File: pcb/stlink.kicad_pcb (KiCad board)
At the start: 4 copper layers, 36.5 x 20 mm, 41 parts, among them J1 USB_A, Q1 S9013, U1 XC6206P332MR, U2 STM32F103C8, Y1 8MHz

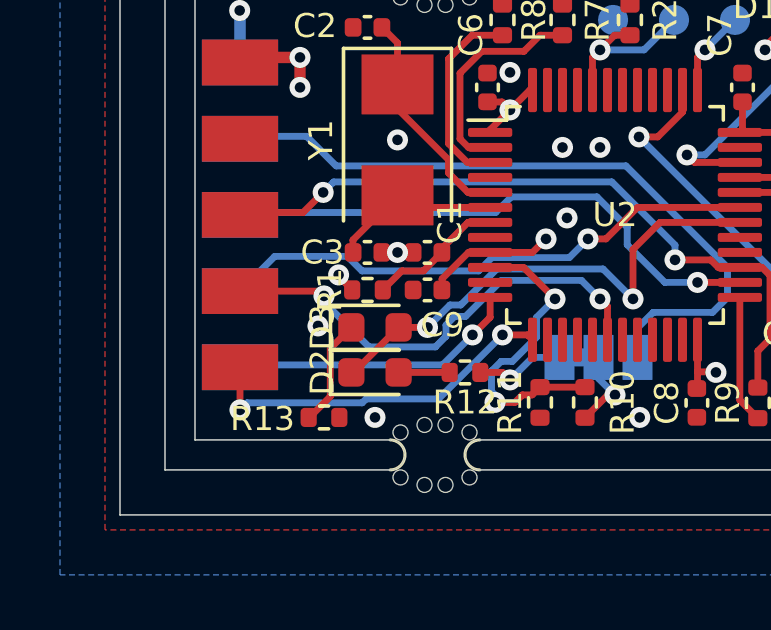
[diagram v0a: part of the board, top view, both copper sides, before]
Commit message: Rev e order
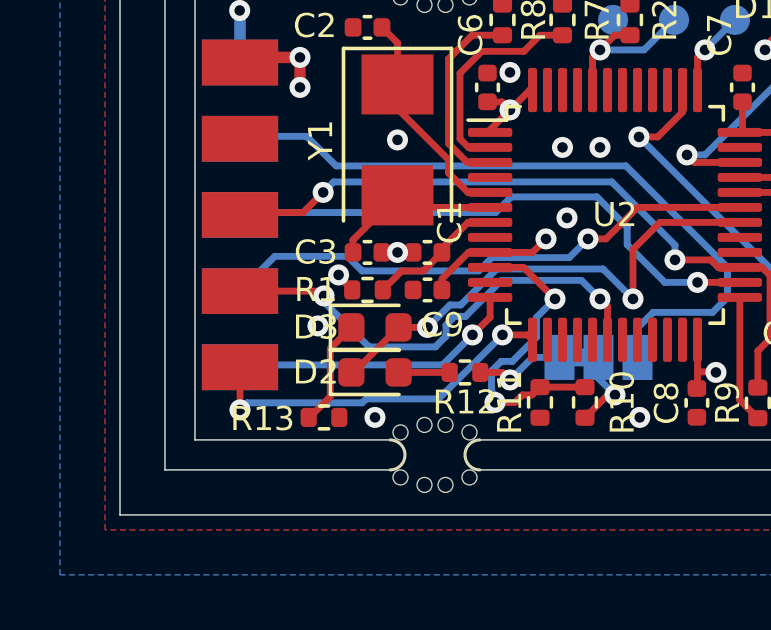
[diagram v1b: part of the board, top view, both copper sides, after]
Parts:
- U2: value STM32F103C8 -> STM32F103CB
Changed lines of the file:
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@@
     )
     (pad_to_mask_clearance 0)
+    (aux_axis_origin 97.13 107.24)
+    (grid_origin 97.09 107.28)
     (pcbplotparams
       (layerselection 0x00010fc_ffffffff)
@@
       (viasonmask false)
       (mode 1)
-      (useauxorigin false)
+      (useauxorigin true)
       (hpglpennumber 1)
       (hpglpenspeed 20)
@@
       (drillshape 0)
       (scaleselection 1)
-      (outputdirectory "stlink_d/")
+      (outputdirectory "stlink_e/")
     )
   )
@@
     (property "Sheetname" "")
     (attr smd)
-    (fp_text reference "C3" (at -1.5 0 unlocked) (layer "F.SilkS")
+    (fp_text reference "C3" (at -1.72 0 unlocked) (layer "F.SilkS")
       (effects (font (size 0.8 0.8) (thickness 0.15)))
     )
@@
     (property "Sheetname" "")
     (attr smd)
-    (fp_text reference "D2" (at -1.75 0 90 unlocked) (layer "F.SilkS")
+    (fp_text reference "D2" (at -1.97 0 unlocked) (layer "F.SilkS")
       (effects (font (size 0.8 0.8) (thickness 0.15)))
     )
@@
     (property "Sheetname" "")
     (attr smd)
-    (fp_text reference "D3" (at -1.75 0 90 unlocked) (layer "F.SilkS")
+    (fp_text reference "D3" (at -1.97 0 unlocked) (layer "F.SilkS")
       (effects (font (size 0.8 0.8) (thickness 0.15)))
     )
@@
     (descr "LQFP, 48 Pin (https://www.analog.com/media/en/technical-documentation/data-sheets/ltc2358-16.pdf), generated with kicad-footprint-generator ipc_gullwing_generator.py")
     (tags "LQFP QFP")
-    (property "LCSC" "C8734")
+    (property "LCSC" "C8304")
     (property "Sheetfile" "stlink.kicad_sch")
     (property "Sheetname" "")
@@
       (effects (font (size 0.8 0.8) (thickness 0.15)))
     )
-    (fp_text value "STM32F103C8" (at 0 5.85) (layer "F.Fab")
+    (fp_text value "STM32F103CB" (at 0 5.85) (layer "F.Fab")
       (effects (font (size 1 1) (thickness 0.15)))
     )
@@
     (property "Sheetname" "")
     (attr smd)
-    (fp_text reference "R1" (at 1.25 0 90 unlocked) (layer "F.SilkS")
-      (effects (font (size 0.8 0.8) (thickness 0.15)))
-    )
+    (fp_text reference "R1" (at 1.72 0 unlocked) (layer "F.SilkS")
+      (effects (font (size 0.8 0.8) (thickness 0.15)))
+    )
